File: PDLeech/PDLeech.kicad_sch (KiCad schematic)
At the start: 12 parts

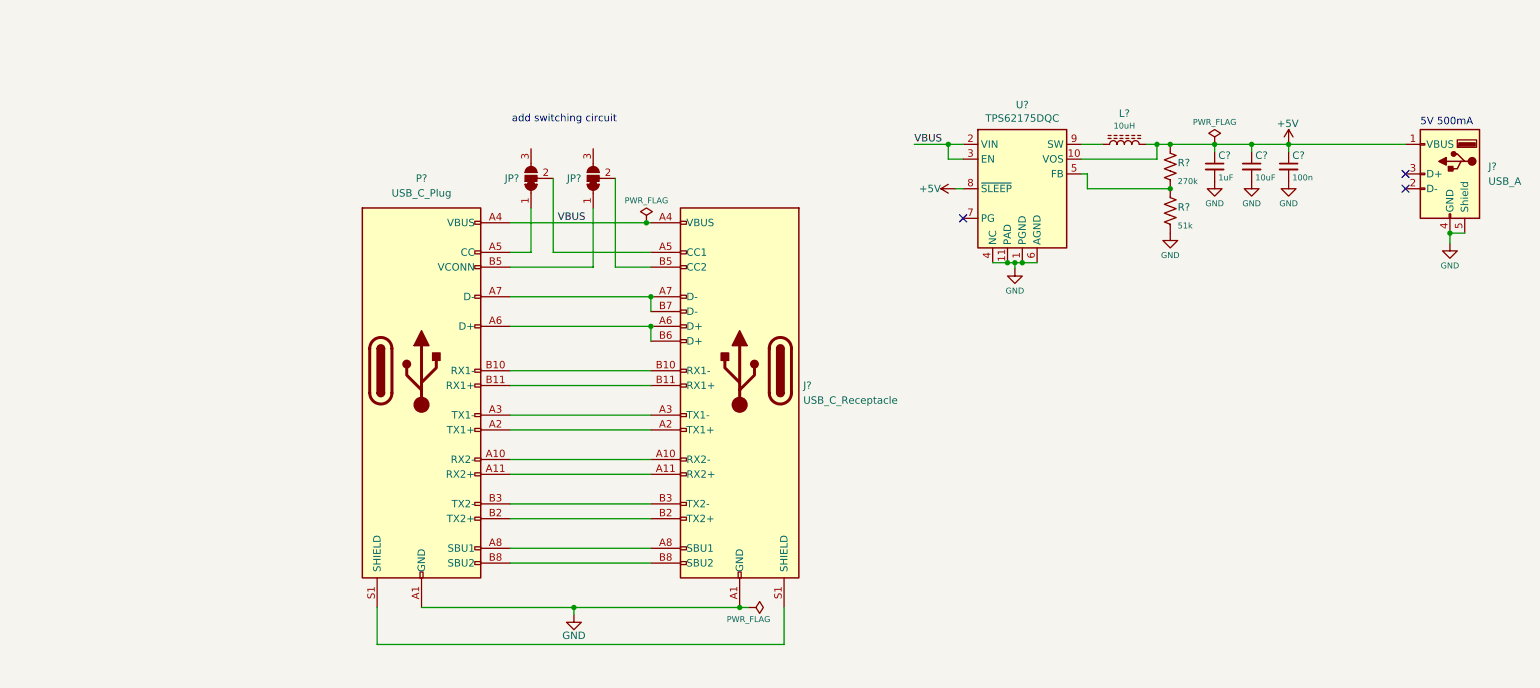
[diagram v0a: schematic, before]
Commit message: schematic finished
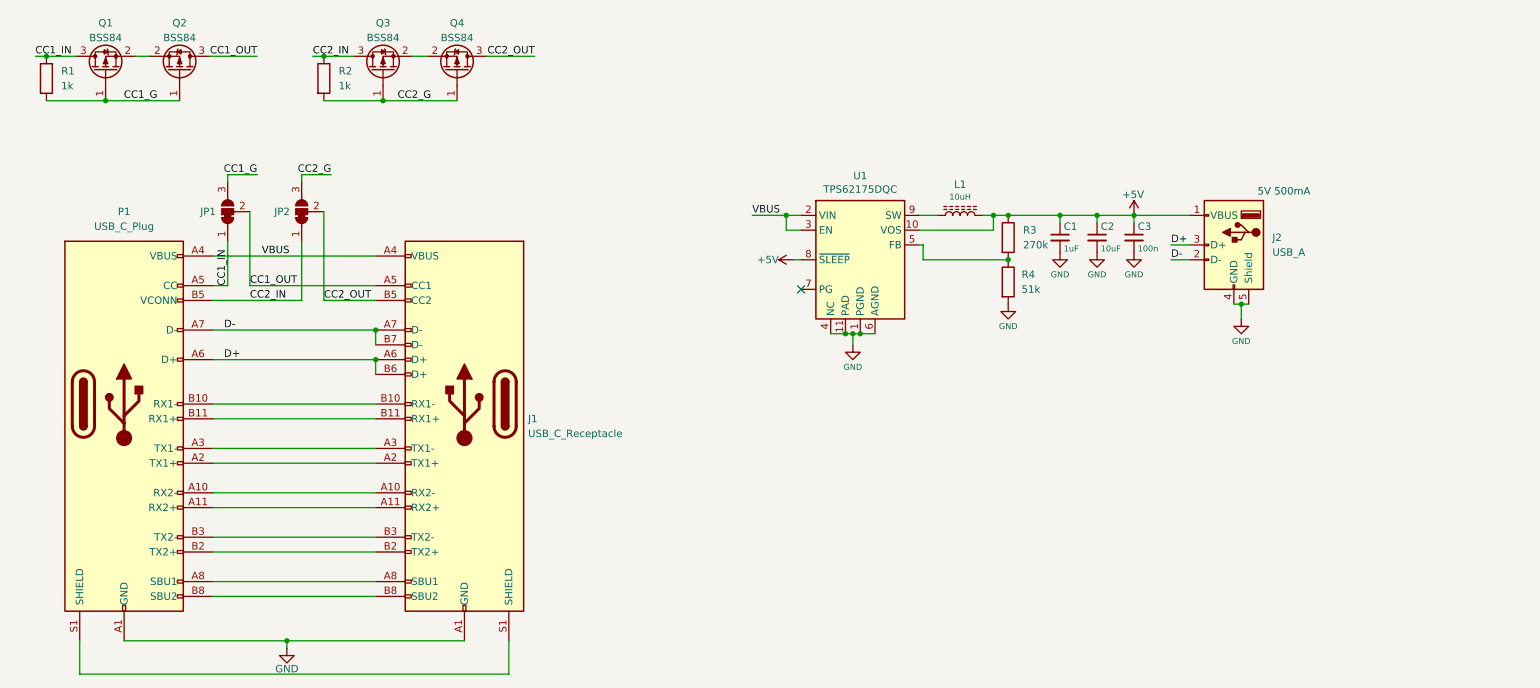
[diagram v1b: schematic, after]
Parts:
- removed R?: 270k, -Passive:R_0603, symbol -Passive:R
- removed R?: 51k, -Passive:R_0603, symbol -Passive:R
- added Q1, Q2, Q3, Q4: BSS84, Package_TO_SOT_SMD:SOT-23, symbol Transistor_FET:BSS84
- added R1, R2: 1k, symbol Device:R
- added R3: 270k, symbol Device:R
- added R4: 51k, symbol Device:R
- gave numbers to parts that had none: 10
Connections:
- net +5V: now also R3.1
- net GND: now also R4.2
- net CC2_IN: now reaches JP2.1 (A), P1.B5 (VCONN)
- net CC2_IN: now also Q3.3 (D), R2.1
- net CC2_OUT: now reaches J1.B5 (CC2), JP2.2 (C)
- net CC2_OUT: now also Q4.3 (D)
- net CC2_G: now reaches JP2.3 (B)
- net CC2_G: now also Q3.1 (G), Q4.1 (G), R2.2
- net at U1.5 (FB): now also R3.2, R4.1
- net CC1_OUT: now reaches J1.A5 (CC1), JP1.2 (C)
- net CC1_OUT: now also Q2.3 (D)
- net D+: now reaches J1.A6 (D+), J1.B6 (D+), P1.A6 (D+)
- net D+: now also J2.3 (D+)
- net D-: now reaches J1.A7 (D-), J1.B7 (D-), P1.A7 (D-)
- net D-: now also J2.2 (D-)
- net CC1_IN: now reaches JP1.1 (A), P1.A5 (CC)
- net CC1_IN: now also Q1.3 (D), R1.1
- net CC1_G: now reaches JP1.3 (B)
- net CC1_G: now also Q1.1 (G), Q2.1 (G), R1.2
- new net: Q1.2 (S), Q2.2 (S)
- new net: Q3.2 (S), Q4.2 (S)
- no-connect marks 3 -> 1
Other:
- note removed: "add switching circuit"
- moved on the sheet: C1, C2, C3, J1, J2, JP1, JP2, L1, P1, U1

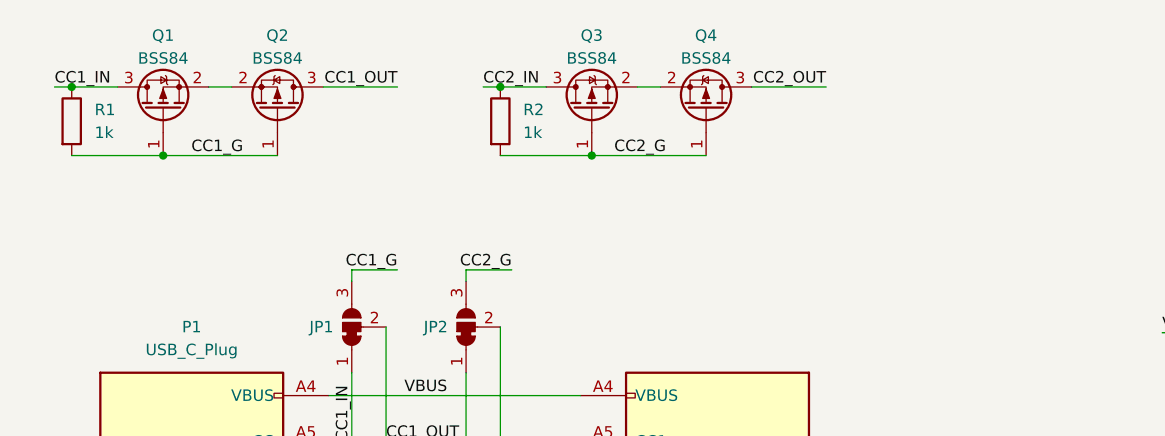
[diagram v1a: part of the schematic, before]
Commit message: updated schematic
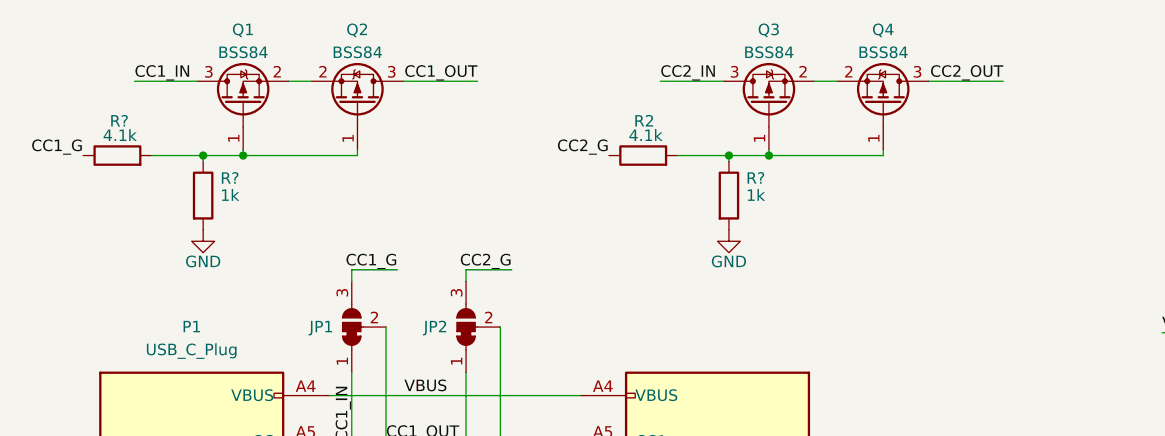
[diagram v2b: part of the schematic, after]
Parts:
- removed R1: 1k, symbol Device:R
- added R?: 4.1k, symbol Device:R
- added R? (x2): 1k, symbol Device:R
- R2: value 1k -> 4.1k
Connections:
- net CC1_G: now also R?.1; no longer Q1.1 (G), Q2.1 (G)
- net CC2_G: now also R2.1; no longer Q3.1 (G), Q4.1 (G), R2.2
- net CC2_IN: no longer R2.1
- net GND: now also R?.2, R?.2
- new net: Q1.1 (G), Q2.1 (G), R?.1, R?.2
- new net: Q3.1 (G), Q4.1 (G), R2.2, R?.1
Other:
- moved on the sheet: Q1, Q2, Q3, Q4, R2
